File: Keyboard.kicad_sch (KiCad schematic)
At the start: 7 parts, among them J1 USB_C_Receptacle, J2 Conn_02x01_Row_Letter_First, U1 ESP32-C3FH4, U4 MAX77301EWAT

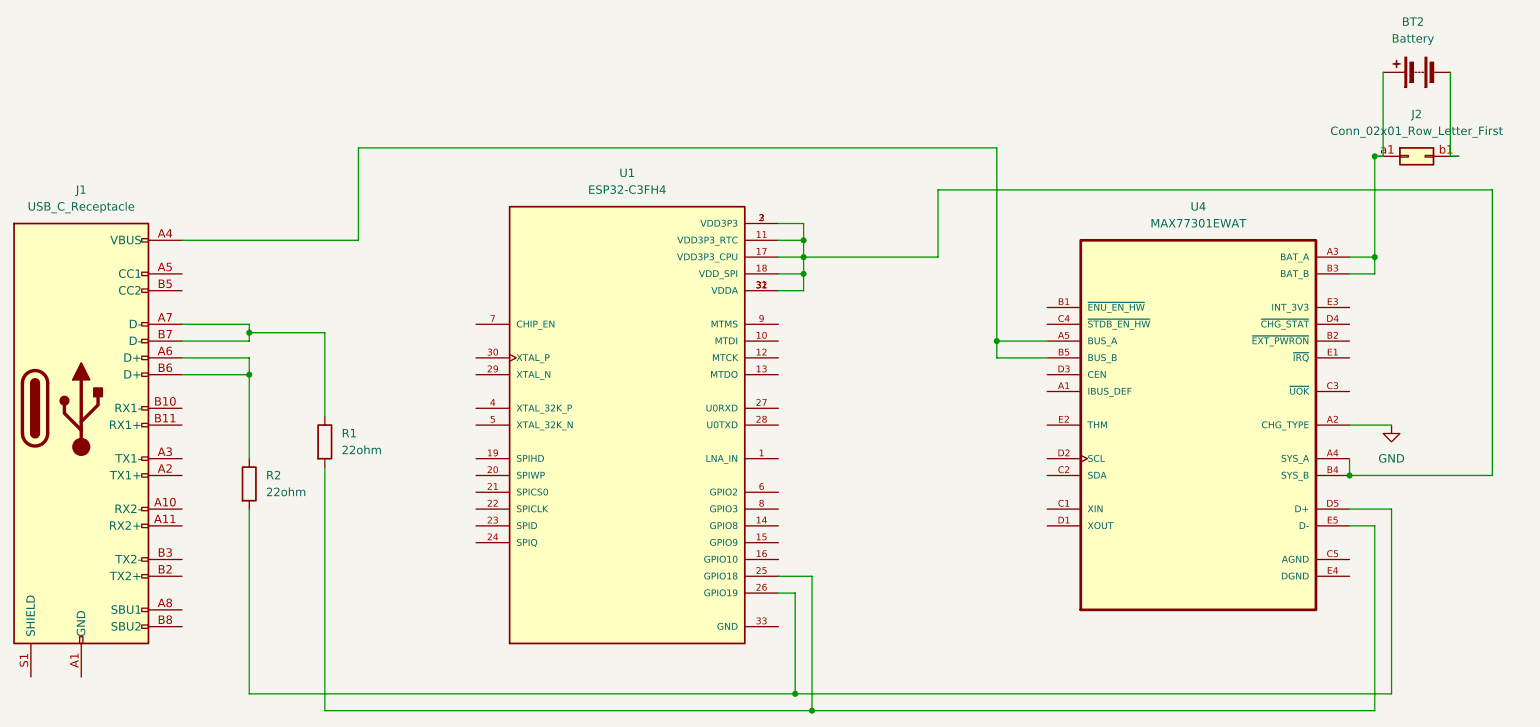
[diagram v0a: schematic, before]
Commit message: some edits
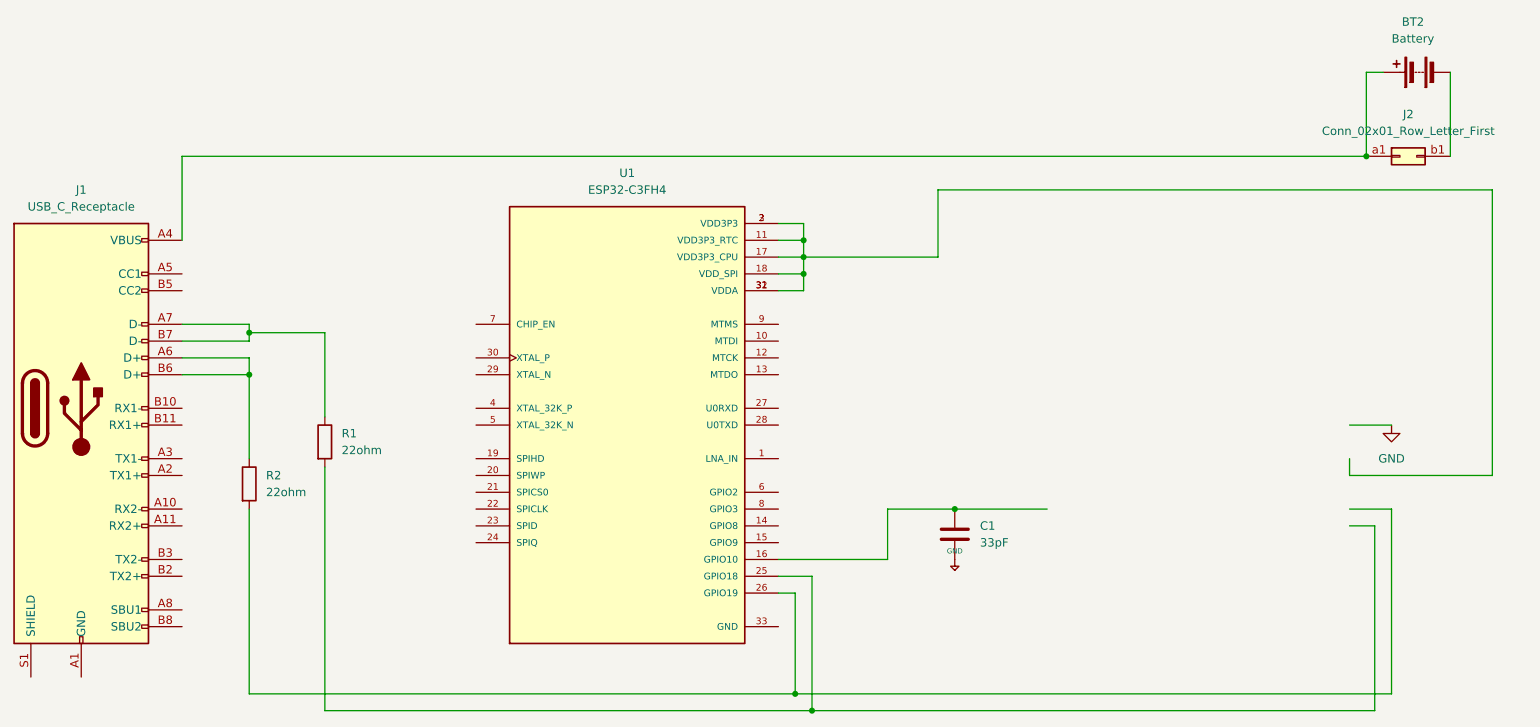
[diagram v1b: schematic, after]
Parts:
- removed U4: MAX77301EWAT, MAX77301EWAT:BGA25N40P5X5_242X242X69N, symbol MAX77301EWAT:MAX77301EWAT
- added C1: 33pF, symbol Device:C
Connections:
- net at BT2.1 (+), J2.a1 (Pin_a1): now also J1.A4 (VBUS), J1.A9 (VBUS), J1.B4 (VBUS), J1.B9 (VBUS)
- net at U1.16 (GPIO10): now also C1.1
- new net +5V: C1.2
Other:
- moved on the sheet: J2
